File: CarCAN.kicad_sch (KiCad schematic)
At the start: 5 parts, among them IC1 TCAN337DCNR, U13 CDSOT23-T24CAN, U14 MCP2515-xST

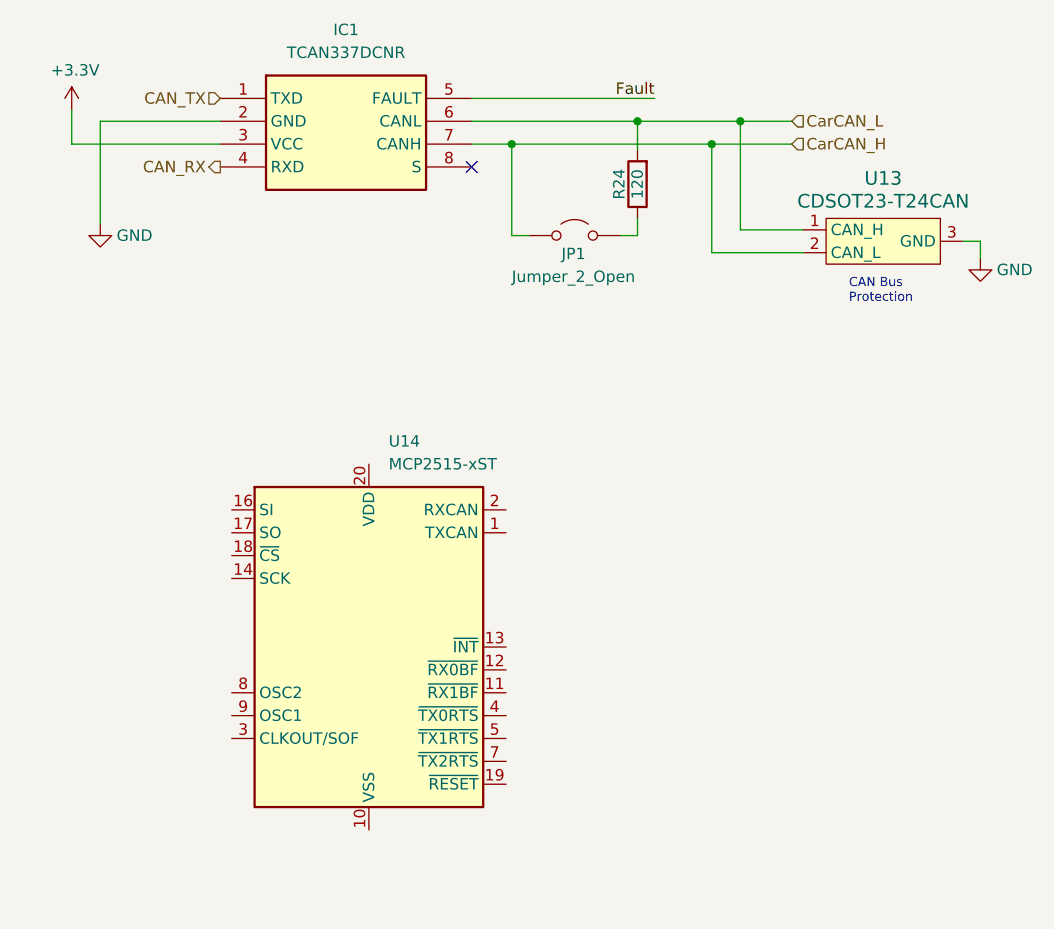
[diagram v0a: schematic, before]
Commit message: worked some more on converting components (unfinished)
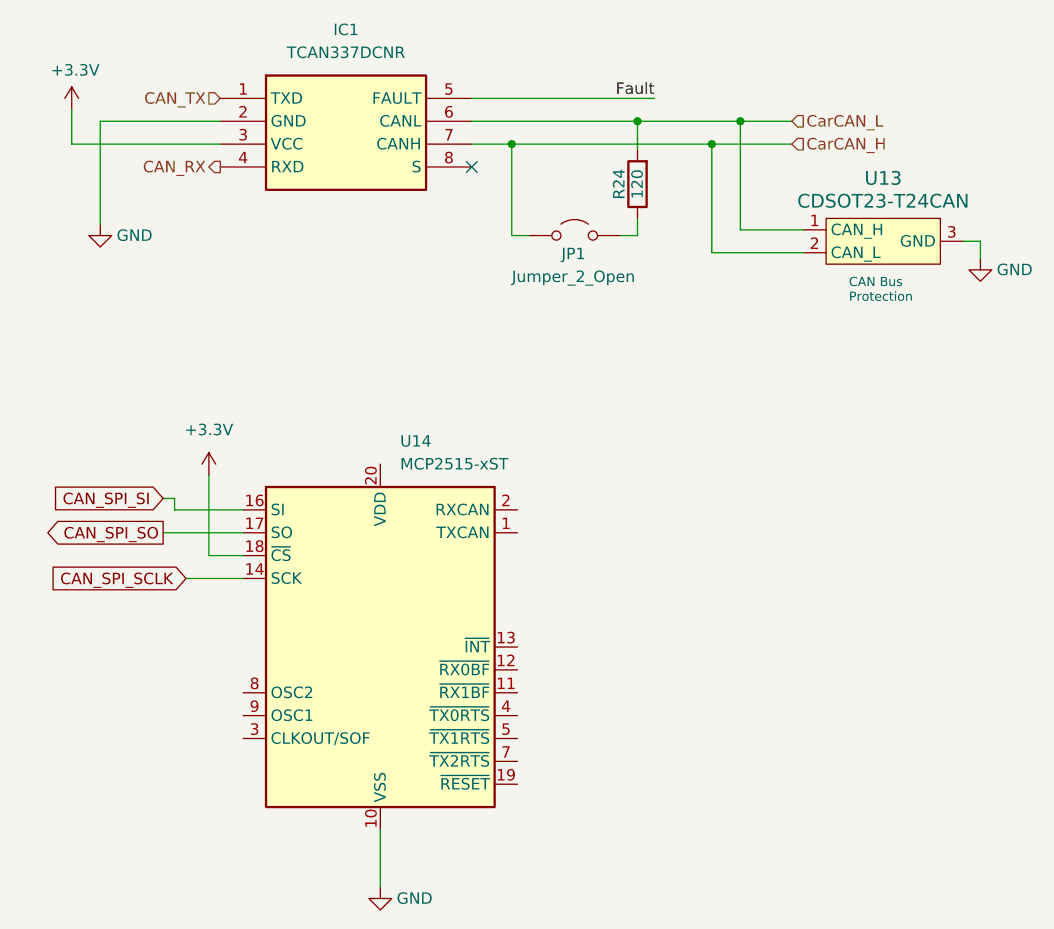
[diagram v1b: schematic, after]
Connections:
- net +3.3V: now also U14.18 (~{CS})
- net GND: now also U14.10 (VSS)
- net CAN_SPI_SCLK: now reaches U14.14 (SCK)
- net CAN_SPI_SI: now reaches U14.16 (SI)
- net CAN_SPI_SO: now reaches U14.17 (SO)
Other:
- moved on the sheet: U14
